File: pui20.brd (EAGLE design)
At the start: 95 x 30 mm, 37 parts, among them IC1 L7805

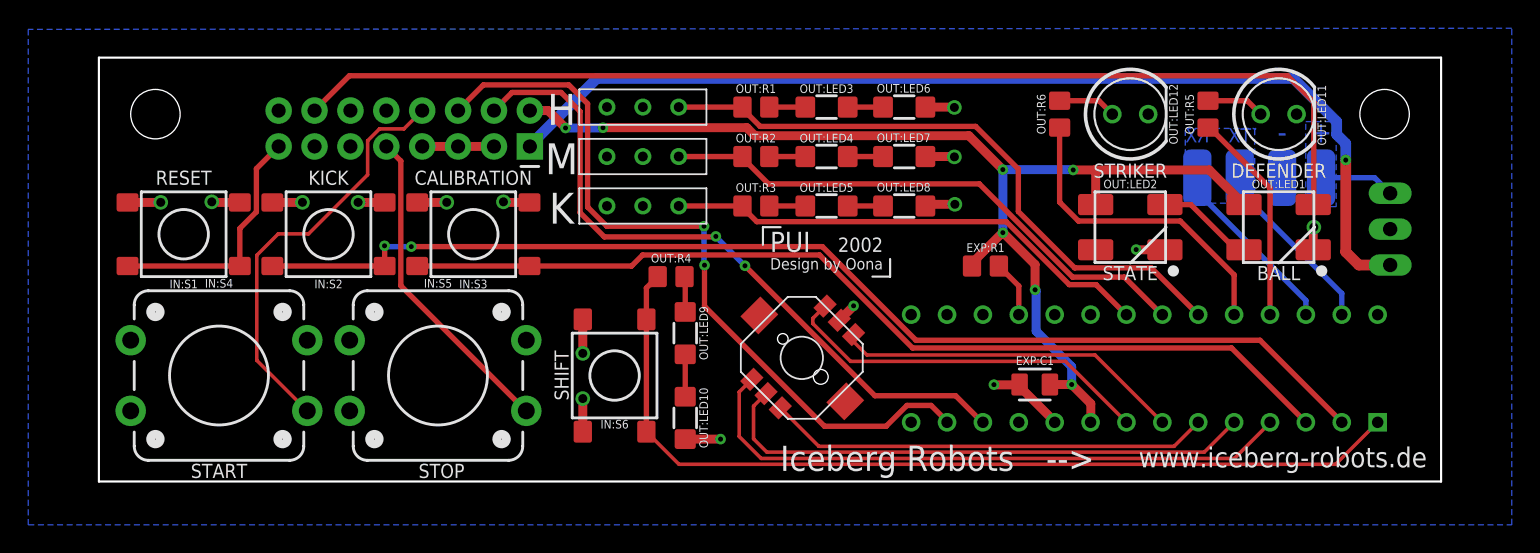
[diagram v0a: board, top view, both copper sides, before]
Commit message: - pui (Corrections)
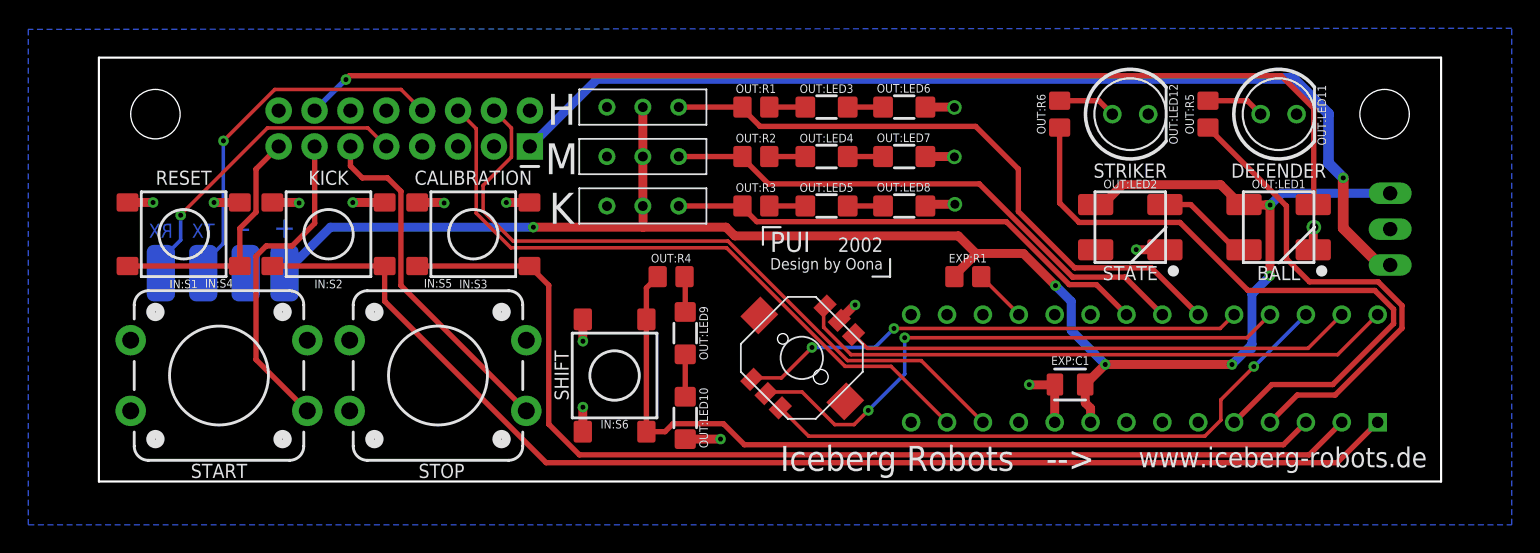
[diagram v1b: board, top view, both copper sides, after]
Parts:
- moved DISPLAY1:GND 73.7 mm to (10.4, 14.7)
- moved DISPLAY1:RX 73.7 mm to (4.39, 14.7)
- moved DISPLAY1:TX 73.7 mm to (7.39, 14.7)
- moved DISPLAY1:VIN 73.7 mm to (13.1, 14.7)
- moved EXP:C1 2.50 mm to (68.7, 6.86)
- moved EXP:R1 1.46 mm to (61.5, 14.5)
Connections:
- net N$4 renamed RESET-B
- net N$5 renamed LED-IN
- removed net EXP:A0: EXP:IC1.15
- removed net EXP:A1: EXP:IC1.16
- removed net EXP:A2: EXP:IC1.17
- removed net EXP:GPA7: EXP:IC1.28
- removed net EXP:NC: EXP:IC1.11
- removed net N$1: X:X1.3, X:X1.5, X:X1.7
- removed net N$11: EXP:IC1.3, IN:S3.A1, IN:S3.A2
- removed net N$12: EXP:IC1.4, IN:U$1.A
- removed net N$13: EXP:IC1.5, IN:U$1.CENTER
- removed net N$14: EXP:IC1.6, IN:U$1.C
- removed net N$15: EXP:IC1.7, IN:U$1.D
- removed net N$16: EXP:IC1.8, IN:U$1.B
- removed net N$18: DISPLAY1:VIN.P$1, IC1.3
- removed net N$2: IN:S4.1, X:X1.8
- removed net N$3: IN:S5.1, X:X1.9
- removed net N$6: EXP:IC1.24, OUT:R6.1
- removed net N$7: EXP:IC1.25, OUT:R5.1
- removed net N$9: EXP:IC1.2, IN:S2.A1, IN:S2.A2
- new net CALIBRATION-B: EXP:IC1.2, IN:S3.A1, IN:S3.A2
- new net CENTER-J: EXP:IC1.25, IN:U$1.CENTER
- new net DEFENCE-LED: EXP:IC1.5, OUT:R6.1
- new net DOWN-J: EXP:IC1.26, IN:U$1.C
- new net KICK-B: EXP:IC1.1, IN:S2.A1, IN:S2.A2
- new net LEFT-J: EXP:IC1.24, IN:U$1.A
- new net RIGHT-J: EXP:IC1.27, IN:U$1.D
- new net START-B: IN:S4.1, X:X1.13
- new net STOP-B: IN:S5.1, X:X1.11
- new net STRIKER-LED: EXP:IC1.4, OUT:R5.1
- new net UP-J: EXP:IC1.28, IN:U$1.B
- net +5V: now also DISPLAY1:VIN.P$1, IC1.3, IN:S7.C, IN:S8.C, IN:S9.C
- net GND: now also EXP:IC1.15, EXP:IC1.16, EXP:IC1.17, EXP:IC1.6, EXP:IC1.7, EXP:IC1.8, X:X1.10, X:X1.12, X:X1.3, X:X1.5, X:X1.7; no longer IN:S7.C, IN:S8.C, IN:S9.C
- net RX: now also X:X1.9; no longer EXP:IC1.26
- net SHIFT-LED: now also EXP:IC1.3; no longer EXP:IC1.1
- net TX: now also X:X1.8; no longer EXP:IC1.27
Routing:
- net KICK-B: track 0.00 -> 86.6 mm
- net N$9: track 82.3 -> 0.00 mm, vias 2 -> 0
- net CALIBRATION-B: track 0.00 -> 77.7 mm
- net N$11: track 68.1 -> 0.00 mm
- net DEFENCE-LED: track 0.00 -> 47.3 mm
- net +5V: track 81.1 -> 124.9 mm, vias 7 -> 6
- net N$12: track 43.7 -> 0.00 mm
- net UP-J: track 0.00 -> 42.7 mm
- net DOWN-J: track 0.00 -> 42.5 mm, vias 0 -> 1
- net CENTER-J: track 0.00 -> 41.4 mm, vias 0 -> 2
- net N$13: track 38.8 -> 0.00 mm
- net LEFT-J: track 0.00 -> 36.0 mm, vias 0 -> 2
- net RIGHT-J: track 0.00 -> 35.9 mm
- net STRIKER-LED: track 0.00 -> 34.8 mm
- net N$14: track 31.4 -> 0.00 mm
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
